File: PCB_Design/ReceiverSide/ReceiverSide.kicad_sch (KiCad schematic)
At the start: 18 parts, among them J1 Conn_01x02_Pin, U1 DRV5053CAQLPGM

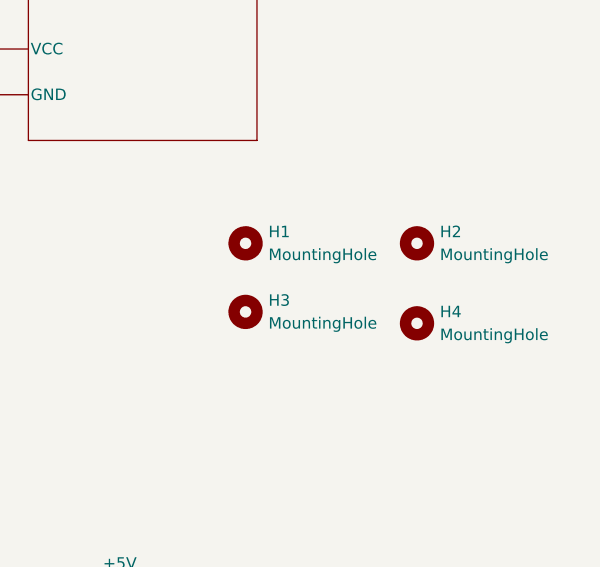
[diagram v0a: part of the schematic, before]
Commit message: fix
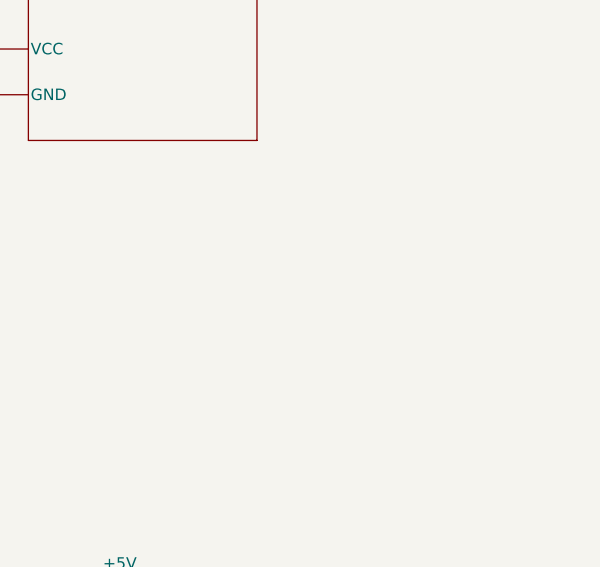
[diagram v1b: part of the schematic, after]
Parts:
- removed H1, H2, H3, H4: MountingHole, MountingHole:MountingHole_3.5mm, symbol Mechanical:MountingHole

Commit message: transmitter pcb
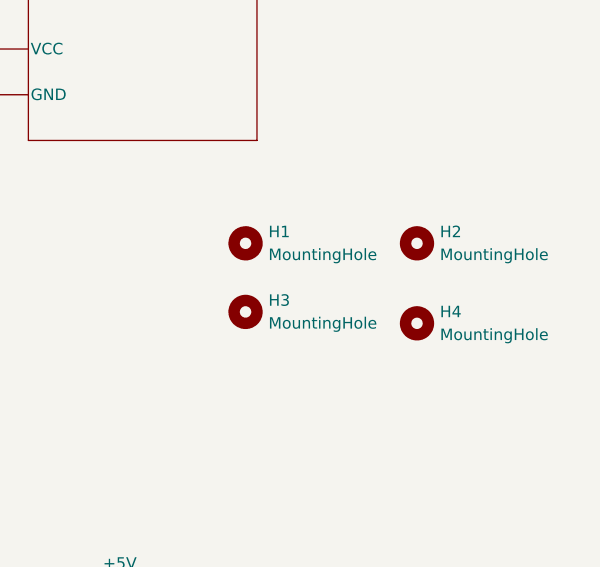
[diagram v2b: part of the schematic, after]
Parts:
- added H1, H2, H3, H4: MountingHole, MountingHole:MountingHole_3.5mm, symbol Mechanical:MountingHole
